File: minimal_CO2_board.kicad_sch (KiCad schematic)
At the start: 1 part, among them U1 ESP32-C3_SUPERMINI

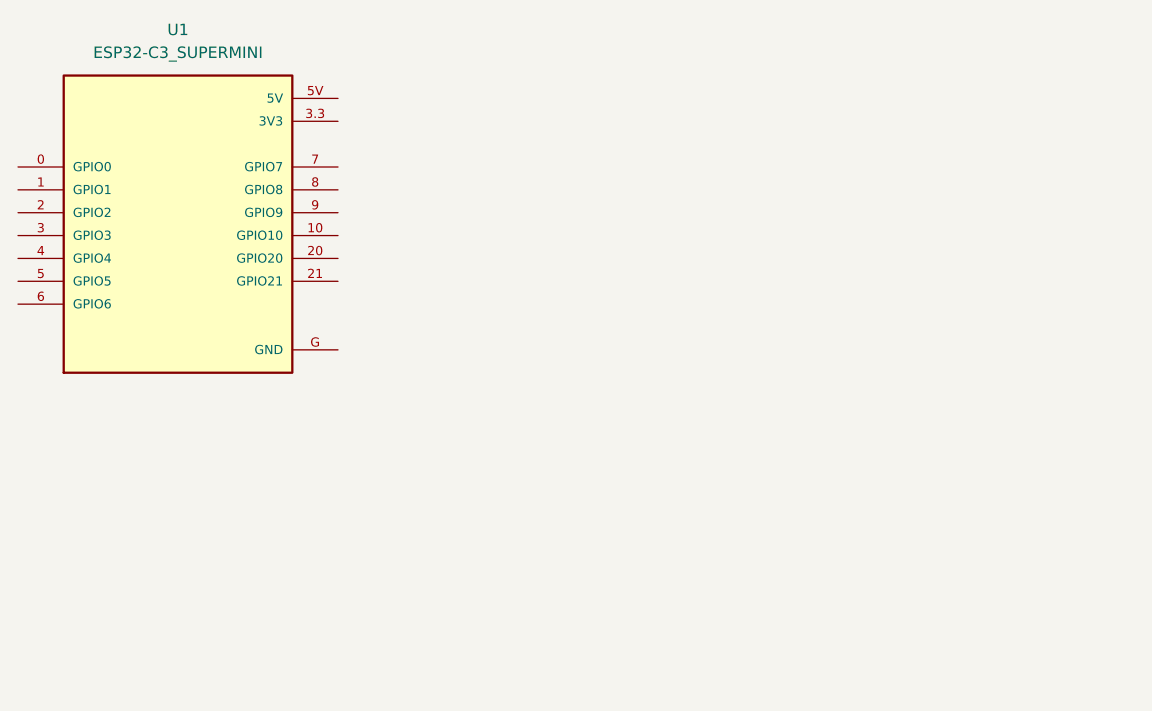
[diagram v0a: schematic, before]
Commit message: changes
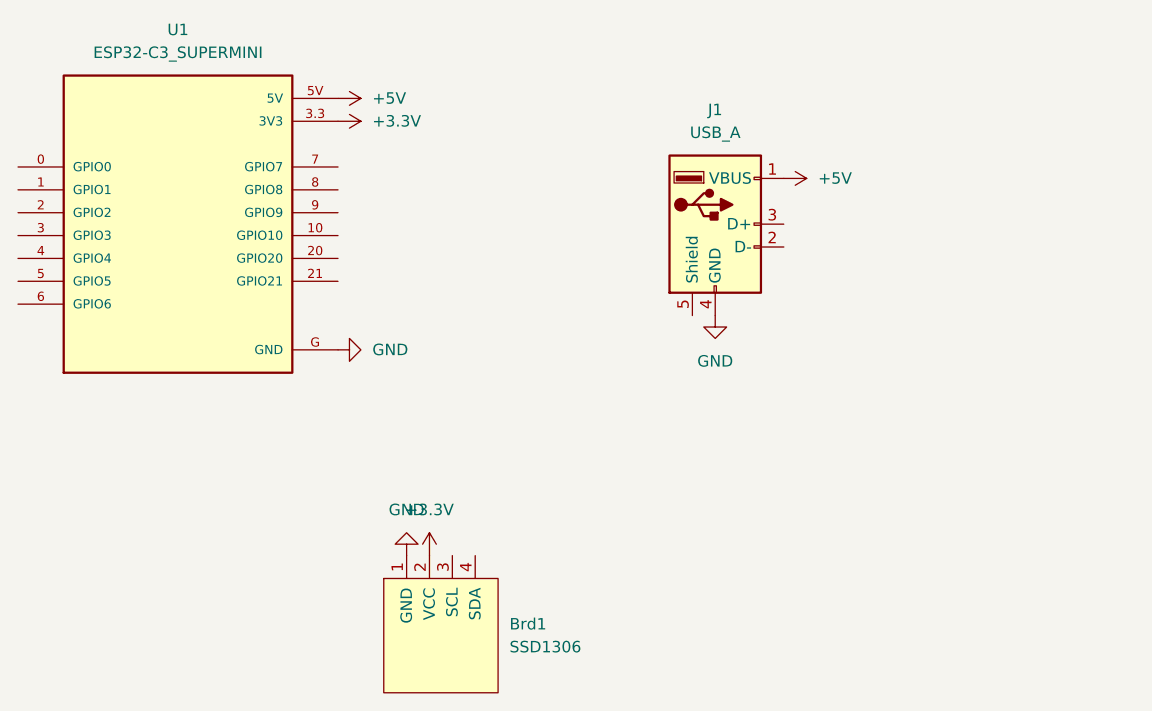
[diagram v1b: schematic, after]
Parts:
- added Brd1: SSD1306, CustomLibrary:128x64OLED, symbol CustomSymbols:SSD1306
- added J1: USB_A, Connector_USB:USB_A_CNCTech_1001-011-01101_Horizontal, symbol Connector:USB_A
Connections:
- net +3.3V: now reaches U1.3.3 (3V3)
- net +3.3V: now also Brd1.2 (VCC)
- net +5V: now reaches U1.5V
- net +5V: now also J1.1 (VBUS)
- net GND: now reaches U1.G (GND)
- net GND: now also Brd1.1 (GND), J1.4 (GND)

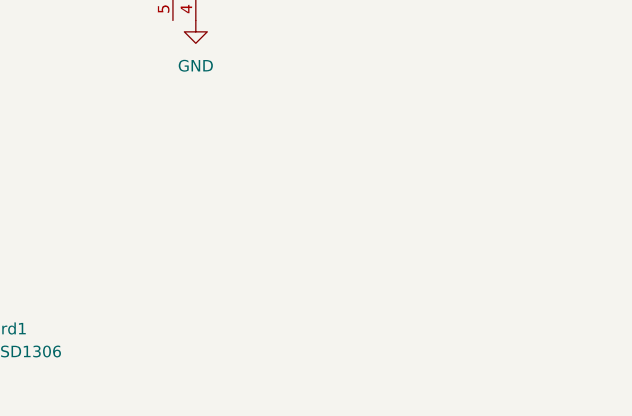
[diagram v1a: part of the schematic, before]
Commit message: update
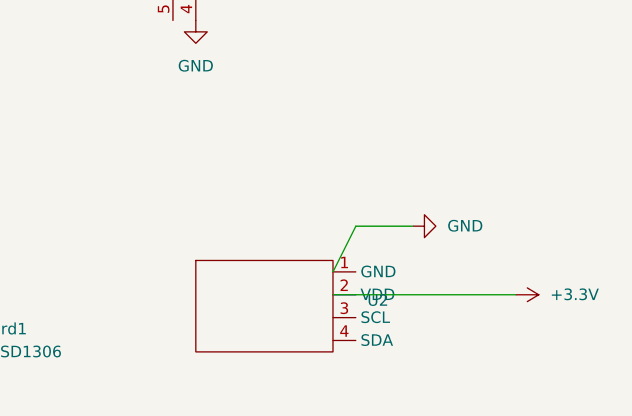
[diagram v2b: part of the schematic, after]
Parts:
- added U2: ~, CustomLibrary:SCD40_CO2_module, symbol CustomSymbols:SCD40_CO2_module
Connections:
- net +3.3V: now also U2.2 (VDD)
- net GND: now also U2.1 (GND)
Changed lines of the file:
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@@
 	(generator_version "9.0")
 	(paper "A4")
+	(wire
+		(pts
+			(xy 147.32 87.63) (xy 140.97 87.63)
+		)
+		(stroke
+			(width 0)
+			(type default)
+		)
+	)
+	(wire
+		(pts
+			(xy 140.97 87.63) (xy 138.43 92.71)
+		)
+		(stroke
+			(width 0)
+			(type default)
+		)
+	)
+	(wire
+		(pts
+			(xy 158.75 95.25) (xy 138.43 95.25)
+		)
+		(stroke
+			(width 0)
+			(type default)
+		)
+	)
 	(symbol
 		(lib_id "power:+5V")
@@
 	)
 	(symbol
+		(lib_id "power:GND")
+		(at 147.32 87.63 90)
+		(unit 1)
+		(exclude_from_sim no)
+		(in_bom yes)
+		(on_board yes)
+		(dnp no)
+		(fields_autoplaced yes)
+		(property "Reference" "#PWR08"
+			(at 153.67 87.63 0)
+			(effects
+				(font
+					(size 1.27 1.27)
+				)
+				(hide yes)
+			)
+		)
+		(property "Value" "GND"
+			(at 151.13 87.6299 90)
+			(effects
+				(font
+					(size 1.27 1.27)
+				)
+				(justify right)
+			)
+		)
+		(property "Footprint" ""
+			(at 147.32 87.63 0)
+			(effects
+				(font
+					(size 1.27 1.27)
+				)
+				(hide yes)
+			)
+		)
+		(property "Datasheet" ""
+			(at 147.32 87.63 0)
+			(effects
+				(font
+					(size 1.27 1.27)
+				)
+				(hide yes)
+			)
+		)
+		(property "Description" "Power symbol creates a global label with name \"GND\" , ground"
+			(at 147.32 87.63 0)
+			(effects
+				(font
+					(size 1.27 1.27)
+				)
+				(hide yes)
+			)
+		)
+		(pin "1"
+		)
+		(instances
+			(project ""
+				(path "/7be59ae3-cff4-4640-882e-dfffcfbe988a"
+					(reference "#PWR08")
+					(unit 1)
+				)
+			)
+		)
+	)
+	(symbol
+		(lib_id "CustomSymbols:SCD40_CO2_module")
+		(at 133.35 90.805 0)
+		(unit 1)
+		(exclude_from_sim no)
+		(in_bom yes)
+		(on_board yes)
+		(dnp no)
+		(fields_autoplaced yes)
+		(property "Reference" "U2"
+			(at 142.24 95.8849 0)
+			(effects
+				(font
+					(size 1.27 1.27)
+				)
+				(justify left)
+			)
+		)
+		(property "Value" "~"
+			(at 142.24 97.79 0)
+			(effects
+				(font
+					(size 1.27 1.27)
+				)
+				(justify left)
+			)
+		)
+		(property "Footprint" "CustomLibrary:SCD40_CO2_module"
+			(at 133.35 90.805 0)
+			(effects
+				(font
+					(size 1.27 1.27)
+				)
+				(hide yes)
+			)
+		)
+		(property "Datasheet" ""
+			(at 133.35 90.805 0)
+			(effects
+				(font
+					(size 1.27 1.27)
+				)
+				(hide yes)
+			)
+		)
+		(property "Description" ""
+			(at 133.35 90.805 0)
+			(effects
+				(font
+					(size 1.27 1.27)
+				)
+				(hide yes)
+			)
+		)
+		(pin "1"
+		)
+		(pin "2"
+		)
+		(pin "3"
+		)
+		(pin "4"
+		)
+		(instances
+			(project ""
+				(path "/7be59ae3-cff4-4640-882e-dfffcfbe988a"
+					(reference "U2")
+					(unit 1)
+				)
+			)
+		)
+	)
+	(symbol
 		(lib_id "power:+3.3V")
 		(at 91.44 91.44 0)
@@
 					(unit 1)
 				)
+			)
+		)
+	)
+	(symbol
+		(lib_id "power:+3.3V")
+		(at 158.75 95.25 270)
+		(unit 1)
+		(exclude_from_sim no)
+		(in_bom yes)
+		(on_board yes)
+		(dnp no)
+		(fields_autoplaced yes)
+		(property "Reference" "#PWR09"
+			(at 154.94 95.25 0)
+			(effects
+				(font
+					(size 1.27 1.27)
+				)
+				(hide yes)
+			)
+		)
+		(property "Value" "+3.3V"
+			(at 162.56 95.2499 90)
+			(effects
+				(font
+					(size 1.27 1.27)
+				)
+				(justify left)
+			)
+		)
+		(property "Footprint" ""
+			(at 158.75 95.25 0)
+			(effects
+				(font
+					(size 1.27 1.27)
+				)
+				(hide yes)
+			)
+		)
+		(property "Datasheet" ""
+			(at 158.75 95.25 0)
+			(effects
+				(font
+					(size 1.27 1.27)
+				)
+				(hide yes)
+			)
+		)
+		(property "Description" "Power symbol creates a global label with name \"+3.3V\""
+			(at 158.75 95.25 0)
+			(effects
+				(font
+					(size 1.27 1.27)
+				)
+				(hide yes)
+			)
+		)
+		(pin "1"
+		)
+		(instances
+			(project ""
+				(path "/7be59ae3-cff4-4640-882e-dfffcfbe988a"
+					(reference "#PWR09")
+					(unit 1)
+				)
